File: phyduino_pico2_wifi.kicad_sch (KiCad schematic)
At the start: 14 parts, among them U11 ESP32-C6-MINI-1, U12 TS3A24159DRC

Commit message: nigthly commit
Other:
- company: (none) -> University of Toronto, Dept. of Physics
- title: (none) -> Phyduino Pico 2
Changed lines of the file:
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@@
 	(generator_version "10.0")
 	(paper "B")
+	(title_block
+		(title "Phyduino Pico 2")
+		(date "2026-05-04")
+		(rev "A")
+		(company "University of Toronto, Dept. of Physics")
+	)
 	(rectangle
 		(start 41.91 88.9)

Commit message: Made schematic changes : merged usb_pd sheet with wifi sheet. made system regulators adjustable.
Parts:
- removed C38: 0.1µF, Capacitor_SMD [KL]:C_0402_1005Metric, symbol Component - Device [KL]:C_Small
- removed TP16, TP17: TestPoint_Small, Component - Test point SMT [UL]:TestPoint_SameSky_CPG-47-TH-B, symbol Connector [KL]:TestPoint_Small
- removed U12: TS3A24159DRC, Package_SON [KL]:Texas_S-PVSON-N10, symbol Analog - Switches - Analog Devices [KL]:TS3A24159DRC
- added C131, C132: 0.1µF, Capacitor_SMD [KL]:C_0402_1005Metric, symbol Device:C_Small
- added C16, C24, C33, C35: 0.1μF, Capacitor_SMD [KL]:C_0805_2012Metric_Pad1.18x1.45mm_HandSolder, symbol Component - Device [KL]:C_Small
- added C17, C18, C25, C27, C36: 22µF, Capacitor_SMD [KL]:C_0805_2012Metric_Pad1.18x1.45mm_HandSolder, symbol Component - Device [KL]:C_Small
- added C19, C23, C29, C32: 10μF, Capacitor_SMD [KL]:C_0805_2012Metric_Pad1.18x1.45mm_HandSolder, symbol Component - Device [KL]:C_Small
- added C28, C9: 0.1µF, Capacitor_SMD [KL]:C_1206_3216Metric_Pad1.33x1.80mm_HandSolder, symbol Component - Device [KL]:C_Small
- added C30: 1µF, Capacitor_SMD [KL]:C_0402_1005Metric, symbol Component - Device [KL]:C_Small
- added C31, C6: 0.1µF, Capacitor_SMD [KL]:C_0402_1005Metric, symbol Component - Device [KL]:C_Small
- added C5, C7: 100pF, Capacitor_SMD [KL]:C_0805_2012Metric_Pad1.18x1.45mm_HandSolder, symbol Component - Device [KL]:C_Small
- added J6, J9: GT-USB-7047A, Connector - PC SMT [UL]:GCT-USBC-GCT_USB4110, symbol KL - Connector:USB_C_Receptacle_USB2.0_16P
- added L1: 6.8µH, Component - Inductor SMT [UL]:L_Bourns_SRP4021HMCT, symbol Inductor - Bourns:L_Bourns_SRP4021HMCT-3R3M
- added L2: 10µH, Component - Inductor SMT [UL]:L_Bourns_SRP4021HMCT, symbol Inductor - Bourns:L_Bourns_SRP4021HMCT-4R7M
- added Q1, Q2: SP30P25NQ, Package_DFN_QFN [KL]:Diodes_UDFN2020-6_Type-F, symbol UL - Transistors - MOSFET:PMPB27EP
- added R10: 5mΩ, Resistor_SMD [KL]:R_0603_1608Metric, symbol Component - Device [KL]:R_Small
- added R11, R12, R7, R8: 5.1kΩ, Resistor_SMD [KL]:R_0402_1005Metric, symbol Component - Device [KL]:R_Small
- added R134: 42.2kΩ, Resistor_SMD [KL]:R_0402_1005Metric, symbol Device:R_Small
- added R135, R138: 21kΩ, Resistor_SMD [KL]:R_0402_1005Metric, symbol Device:R_Small
- added R136, R137: 5.1kΩ, Resistor_SMD [KL]:R_0402_1005Metric, symbol Device:R_Small
- added R139, R141: 154kΩ, Resistor_SMD [KL]:R_0402_1005Metric, symbol Device:R_Small
- added R140, R143, R144: 39.2kΩ, Resistor_SMD [KL]:R_0402_1005Metric, symbol Device:R_Small
- added R142, R145: 10kΩ, Resistor_SMD [KL]:R_0402_1005Metric, symbol Device:R_Small
- added R37, R47, R48: 5.1kΩ, Resistor_SMD [KL]:R_0402_1005Metric, symbol phyduino_pico:R_Small
- added R40, R41: 100Ω, Resistor_SMD [KL]:R_0402_1005Metric, symbol phyduino_pico:R_Small
- added R51: 47kΩ, Resistor_SMD [KL]:R_0805_2012Metric_Pad1.20x1.40mm_HandSolder, symbol phyduino_pico:R_Small
- added R52: 16.5kΩ, Resistor_SMD [KL]:R_0805_2012Metric_Pad1.20x1.40mm_HandSolder, symbol phyduino_pico:R_Small
- added R53: 111kΩ, Resistor_SMD [KL]:R_0805_2012Metric_Pad1.20x1.40mm_HandSolder, symbol phyduino_pico:R_Small
- added R54: 18.7kΩ, Resistor_SMD [KL]:R_0805_2012Metric_Pad1.20x1.40mm_HandSolder, symbol phyduino_pico:R_Small
- added R56: 196kΩ, Resistor_SMD [KL]:R_0805_2012Metric_Pad1.20x1.40mm_HandSolder, symbol phyduino_pico:R_Small
- added R57: 62kΩ, Resistor_SMD [KL]:R_0805_2012Metric_Pad1.20x1.40mm_HandSolder, symbol phyduino_pico:R_Small
- added R58: 157kΩ, Resistor_SMD [KL]:R_0805_2012Metric_Pad1.20x1.40mm_HandSolder, symbol phyduino_pico:R_Small
- added R59: 30kΩ, Resistor_SMD [KL]:R_0805_2012Metric_Pad1.20x1.40mm_HandSolder, symbol phyduino_pico:R_Small
- added R6, R9: 220kΩ, Resistor_SMD [KL]:R_0805_2012Metric_Pad1.20x1.40mm_HandSolder, symbol Component - Device [KL]:R_Small
- added TH1: 10kΩ@25°C, Resistor_SMD [KL]:R_0402_1005Metric, symbol Component - Device [KL]:Thermistor_NTC
- added TP10, TP11, TP13, TP18, TP2, TP22, TP4, TP5, TP6, TP7: TestPoint_Small, Component - Test point SMT [UL]:TestPoint_SameSky_CPG-47-TH-B, symbol Connector [KL]:TestPoint_Small
- added U10, U8: AP63200WU, Package_TO_SOT_SMD [KL]:TSOT-23-6_HandSoldering, symbol Power - Switching Regulator [KL]:AP63200WU
- added U108, U109: TPS2121RUXR, Package - QFN [UL]:VQFN-HR-12, symbol PMIC - TI:TPS2121RUX
- added U6: AP33772SDKZ-13-FA02, Package_DFN_QFN [KL]:QFN-24-1EP_4x4mm_P0.5mm_EP2.75x2.75mm, symbol Interface - USB:AP33772S
- added U9: TPUSBLC6-2P6, Package_TO_SOT_SMD [KL]:SOT-666, symbol Protection - Signal:USBLC6-2P6
- added Z3: ESDA25P35-1U1M-ES, Diode_SMD [KL]:ST_QFN-2L_1.6x1.0mm, symbol phyduino_pico:D_Zener_Filled
- U11: value ESP32-C6-MINI-1 -> ESP32-C6-MINI-1-H4
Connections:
- net WIFI_UART_RX is gone; now on net WIFI_DL_UART_RX: TP9.1
- net WIFI_UART_TX is gone; now on net WIFI_DL_UART_TX: TP8.1
- net +3.3V: now also C17.1, C18.1, C5.1, L1.2, R56.1, R7.1, R8.1, U9.5 (VBUS)
- net GND: now also C131.2, C132.2, C17.2, C18.2, C19.2, C23.2, C25.2, C27.2, C28.2, C29.2, C30.1, C31.1, C32.2, C33.2, C35.2, C36.2, C6.1, C9.2, J6.A1 (GND), J6.A12 (GND), J6.B1 (GND), J6.B12 (GND), J9.A1 (GND), J9.A12 (GND), J9.B1 (GND), J9.B12 (GND), R11.2, R12.2, R134.1, R136.1, R137.1, R143.1, R144.1, R145.1, R47.2, R48.2, R52.2, R54.2, R57.2, R59.2, R6.2, R9.2, TH1.2, U10.4 (GND), U108.12 (GND), U108.3 (CP2), U108.6 (PR1), U108.9 (ST), U109.12 (GND), U6.25 (EP), U6.3 (GND), U8.4 (GND), U9.2 (GND), Z3.2 (A)
- net WIFI_AT_UART_CTS: now reaches U11.10 (IO5)
- net XTAL_32K_P: now reaches U11.12 (IO0)
- net XTAL_32K_N: now reaches U11.13 (IO1)
- net WIFI_AT_UART_RX: now reaches U11.15 (IO6)
- net WIFI_AT_UART_RX: now also R55.2
- net WIFI_AT_UART_TX: now reaches U11.16 (IO7)
- net WIFI_AT_UART_RTS: now reaches U11.9 (IO4)
- net AT_UART_RX: no longer names the net of U11.25 (IO19)
- net AT_UART_RX: no longer R55.2
- net AT_UART_TX: no longer names the net of U11.28 (IO22)
- net DL_UART_RX renamed WIFI_DL_UART_RX
- net DL_UART_TXD renamed WIFI_DL_UART_TX
- net WIFI_UART_CTS: no longer names the net of U11.20 (IO15)
- net WIFI_UART_RTS: no longer names the net of U11.19 (IO14)
- new net: J9.A6 (D+), J9.B6 (D+)
- new net: J9.A7 (D-), J9.B7 (D-)
- new net: R40.1, R41.2
- new net: U6.10 (NC), U6.14 (NC), U6.2 (NC), U6.21 (NC)
- new net +5.0V: U108.1 (OUT), U108.8 (OUT)
- new net +5.0V_DCDC: C25.1, C36.1, C7.1, L2.2, R135.2, R58.1, TP22.1, U108.7 (IN1)
- new net +VUSB: C19.1, C23.1, R138.2, R51.1, R53.1, TP13.1, U10.3 (IN), U108.2 (IN2), U109.1 (OUT), U109.8 (OUT), U8.3 (IN)
- new net +VUSB_COMM: C27.1, J6.A4 (VBUS), J6.A9 (VBUS), J6.B4 (VBUS), J6.B9 (VBUS), R139.2, TP18.1, U109.7 (IN1)
- new net +VUSB_PD: C29.1, C33.1, J9.A4 (VBUS), J9.A9 (VBUS), J9.B4 (VBUS), J9.B9 (VBUS), R10.1, U6.1 (ISENP), Z3.1 (K)
- new net +VUSB_PD_OUT: C32.1, C35.1, Q2.1 (D), Q2.2 (D), Q2.5 (D), Q2.6 (D), Q2.7 (D), R141.2, R41.1, TP11.1, U109.2 (IN2)
- new net DCDC_3V3_BST: C16.1, U8.6 (BST)
- new net DCDC_3V3_EN: R51.2, R52.1, U8.2 (EN)
- new net DCDC_3V3_FB: C5.2, R56.2, R57.1, U8.1 (FB)
- new net DCDC_3V3_SW: C16.2, L1.1, U8.5 (SW)
- new net DCDC_5V0_BST: C24.1, U10.6 (BST)
- new net DCDC_5V0_EN: R53.2, R54.1, U10.2 (EN)
- new net DCDC_5V0_FB: C7.2, R58.2, R59.1, U10.1 (FB)
- new net DCDC_5V0_SW: C24.2, L2.1, U10.5 (SW)
- new net I2C1_SCL: R7.2, U6.5 (SCL)
- new net I2C1_SDA: R8.2, U6.4 (SDA)
- new net PMUX_LIM: R134.2, U108.10 (ILM)
- new net PMUX_OV1: R135.1, R136.2, U108.5 (OV1)
- new net PMUX_OV2: R137.2, R138.1, U108.4 (OV2)
- new net PMUX_SS: C131.1, U108.11 (SS)
- new net PSW_STATUS: U109.9 (ST)
- new net USBPD_CC1: J9.A5 (CC1), R11.1, TP4.1, U6.17 (CC1)
- new net USBPD_CC2: J9.B5 (CC2), R12.1, TP6.1, U6.16 (CC2)
- new net USBPD_FLIP: U6.6 (FLIP)
- new net USBPD_GPIO: U6.7 (GPIO)
- new net USBPD_IFB: C31.2, U6.15 (IFB)
- new net USBPD_INT: U6.9 (INT)
- new net USBPD_OTP: TH1.1, U6.13 (OTP)
- new net USBPD_PROT_GATE: Q1.3 (G), Q2.3 (G), R37.1
- new net USBPD_PROT_SOURCE_DRAIN: Q1.4 (S), Q1.8 (S), Q2.4 (S), Q2.8 (S), TP5.1
- new net USBPD_PWR_EN: R37.2, TP10.1, U6.23 (PWR_EN)
- new net USBPD_V18: C6.2, U6.12 (V18)
- new net USBPD_V5V: C30.2, U6.20 (V5V)
- new net USBPD_VCC: Q1.1 (D), Q1.2 (D), Q1.5 (D), Q1.6 (D), Q1.7 (D), R10.2, TP2.1, U6.24 (VCC)
- new net USBPD_VOUT: R40.2, TP7.1, U6.22 (VOUT)
- new net USB_CC1: J6.A5 (CC1), R48.1
- new net USB_CC2: J6.B5 (CC2), R47.1
- new net USB_COM_D_N: J6.A7 (D-), J6.B7 (D-), U9.4 (I/O2)
- new net USB_COM_D_P: J6.A6 (D+), J6.B6 (D+), U9.6 (I/O1)
- new net USB_COM_SHIELD: C9.1, J6.S1 (SH), R6.1
- new net USB_D_N: U9.3 (I/O2)
- new net USB_D_P: U9.1 (I/O1)
- new net USB_PD_SHIELD: C28.1, J9.S1 (SH), R9.1
- new net USB_PMUX_CP2: R141.1, R142.2, U109.3 (CP2)
- new net USB_PMUX_LIM: R143.2, U109.10 (ILM)
- new net USB_PMUX_OV1: R140.1, R145.2, U109.5 (OV1)
- new net USB_PMUX_OV2: R142.1, R144.2, U109.4 (OV2)
- new net USB_PMUX_PR1: R139.1, R140.2, U109.6 (PR1)
- new net USB_PMUX_SS: C132.1, U109.11 (SS)
- no-connect marks 14 -> 28
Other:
- note added: "- 2.4GHz Wi-Fi 6 & BLE 5.0"
- note added: "- Both modules are pin compatiable, either can be used."
- note added: "- ESP-AT version 4.1.1.0"
- note added: "- ESP-AT version 5.0.1.0"
- note added: "- GitHub fork repo for ESP-AT: https://github.com/perc-sw/esp-at"
- note added: "- Hardware connection guide : https://docs.espressif.com/projects/esp-at/en/latest/esp32c6/Get_Started/Hardware_connection.html"
- note added: "- Hardware connection guide : https://docs.espressif.com/projects/esp-at/en/latest/esp32c61/Get_Started/Hardware_connection.html"
- note added: "- J6 Only provides +5.0V (3A) power and USB 2.0 communication."
- note added: "- J9 can negoiate +5.0V to 20.0V with current ouput varying form 100mA to 5.0A"
- note added: "- Not for low power applications."
- note added: "- To download ESP-AT firmware to ESP32 module use UART0 pins (TXD0 & RXD0)."
- note added: "- U10 will only enable when +VUSB is above +7.0V."
- note added: "- U108 select between +VUSB and the output of U10. If both voltages are below +5.5V, U10's output will be selected."
- note added: "- U109 will select which input power gets used. +VUSB_PD has priority if present."
- note added: "- U8 will only enable when +VUSB is above +4.3V."
- note added: "- Using ESP-AT as the network interface API."
- note added: ">1.06V"
- note added: "ESP32-C6-MINI-1:"
- note added: "ESP32-C61-MINI-1:"
- note added: "I^{2}C Addr = 0x52"
- note added: "I_{LIMIT} = 2.6A"
- note added: "I_{LIMIT} = 2.7A"
- note added: "Low=Disable, High=Enable"
- note added: "NOTES:"
- note added: "Over Voltage Protection = 22V"
- note added: "Over Voltage Protection= 5.5V"
- note added: "Required Hardware connections"
- note added: "System Power Regulators"
- note added: "UART/USB Firmware download"
- note added: "USB Power Delivery"
- note added: "V_{EN}=4.3V"
- note added: "V_{EN}=7.0V"
- note added: "V_{OVER} = 5.5V"
- note added: "WiFi Module Interface"
- moved on the sheet: C13, C37, R44, R45, R50, R55, TP14, TP8, TP9, U11

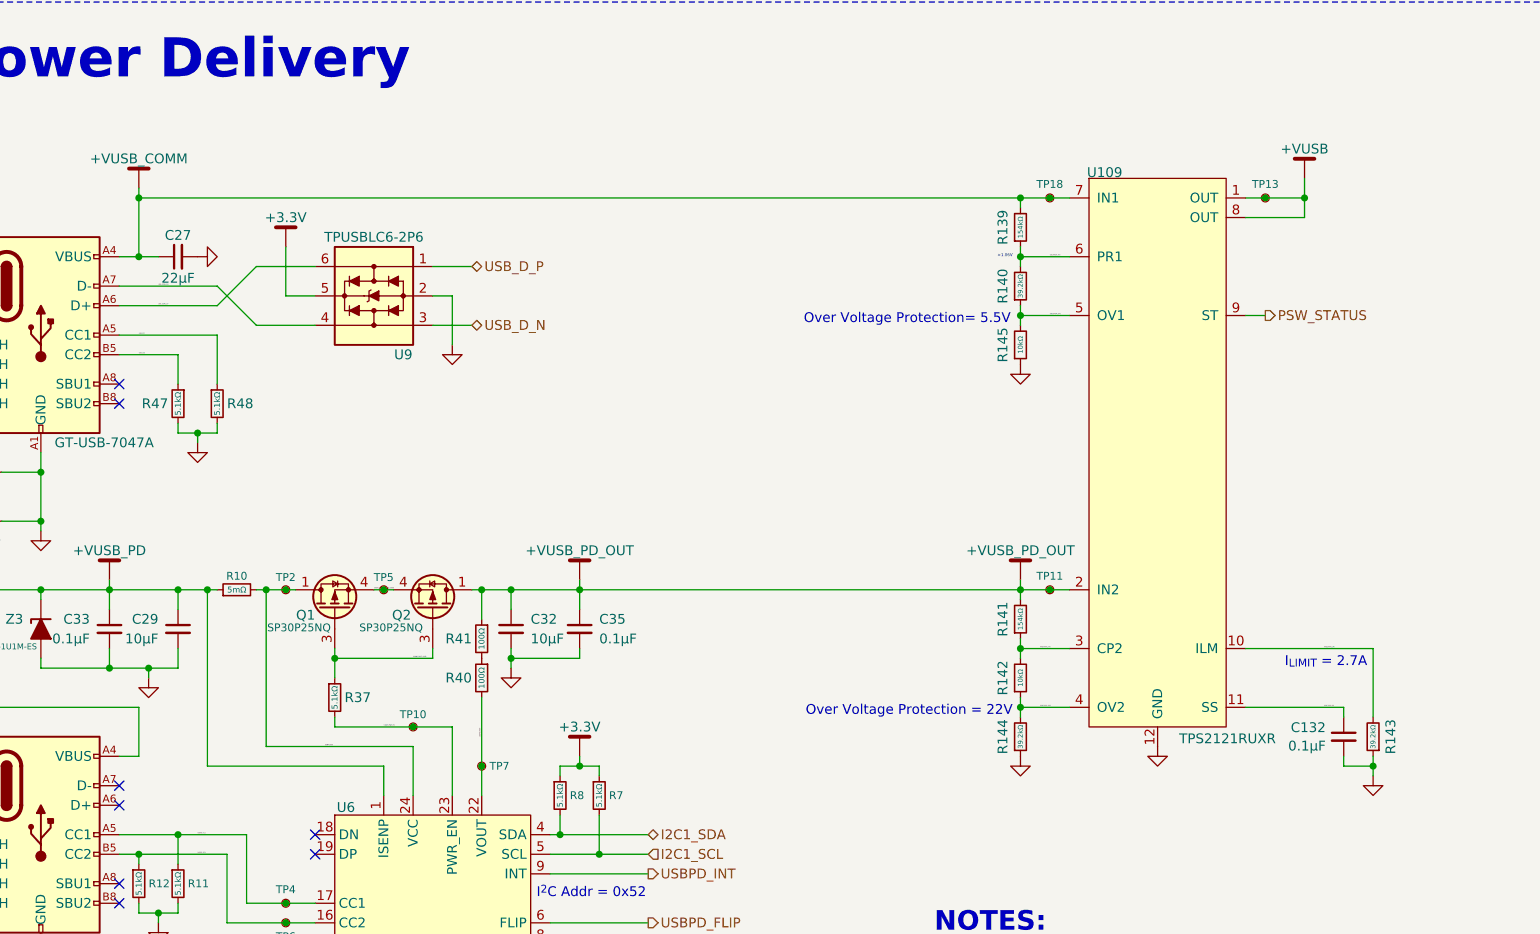
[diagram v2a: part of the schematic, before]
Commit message: development update.
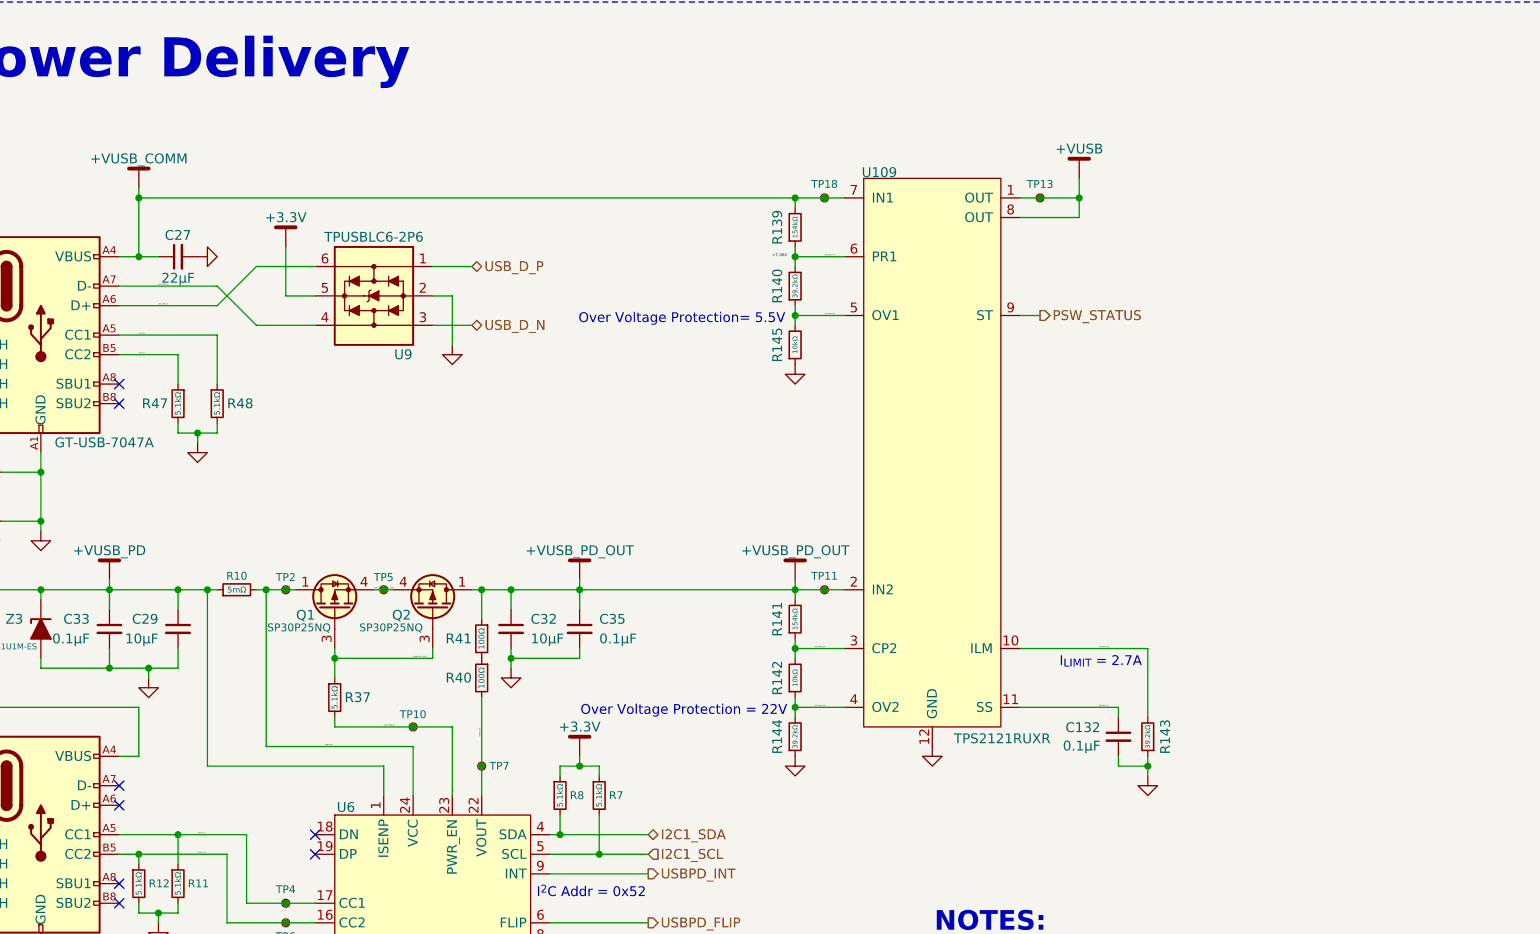
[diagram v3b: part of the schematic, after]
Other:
- moved on the sheet: C132, R139, R140, R141, R142, R143, R144, R145, TP11, TP13, TP18, U109
